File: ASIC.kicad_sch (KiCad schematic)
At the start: 66 parts, among them U10 BM1370_mode1, U11 MCP1824T-1202E/OT, U12 MCP1824T-0802E, U7 SN74AVC4T774, U8 25MHz, U9 BM1370_mode1

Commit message: More BOM cleanup
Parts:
- C38, C54, C55, C56, C57, C58, C59, C60, C61, C62: DK 490-5523-1-ND -> 490-18214-1-ND
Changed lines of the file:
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@@
 			)
 		)
-		(property "DK" "490-5523-1-ND"
+		(property "DK" "490-18214-1-ND"
 			(at 231.14 72.39 0)
 			(effects
@@
 			)
 		)
-		(property "DK" "490-5523-1-ND"
+		(property "DK" "490-18214-1-ND"
 			(at 222.25 72.39 0)
 			(effects
@@
 			)
 		)
-		(property "DK" "490-5523-1-ND"
+		(property "DK" "490-18214-1-ND"
 			(at 240.03 72.39 0)
 			(effects
@@
 			)
 		)
-		(property "DK" "490-5523-1-ND"
+		(property "DK" "490-18214-1-ND"
 			(at 118.11 72.39 0)
 			(effects
@@
 			)
 		)
-		(property "DK" "490-5523-1-ND"
+		(property "DK" "490-18214-1-ND"
 			(at 142.24 72.39 0)
 			(effects
@@
 			)
 		)
-		(property "DK" "490-5523-1-ND"
+		(property "DK" "490-18214-1-ND"
 			(at 109.22 72.39 0)
 			(effects
@@
 			)
 		)
-		(property "DK" "490-5523-1-ND"
+		(property "DK" "490-18214-1-ND"
 			(at 213.36 72.39 0)
 			(effects
@@
 			)
 		)
-		(property "DK" "490-5523-1-ND"
+		(property "DK" "490-18214-1-ND"
 			(at 246.38 72.39 0)
 			(effects
@@
 			)
 		)
-		(property "DK" "490-5523-1-ND"
+		(property "DK" "490-18214-1-ND"
 			(at 127 72.39 0)
 			(effects
@@
 			)
 		)
-		(property "DK" "490-5523-1-ND"
+		(property "DK" "490-18214-1-ND"
 			(at 135.89 72.39 0)
 			(effects

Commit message: change config resistors for TPS546 regulator
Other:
- title: (none) -> Bitaxe Gamma Turbo
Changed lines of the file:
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@@
 	(generator "eeschema")
 	(generator_version "8.0")
-	(paper "A4")
+	(paper "A3")
+	(title_block
+		(title "Bitaxe Gamma Turbo")
+		(rev "800")
+	)
 	(junction
 		(at 127 68.58)

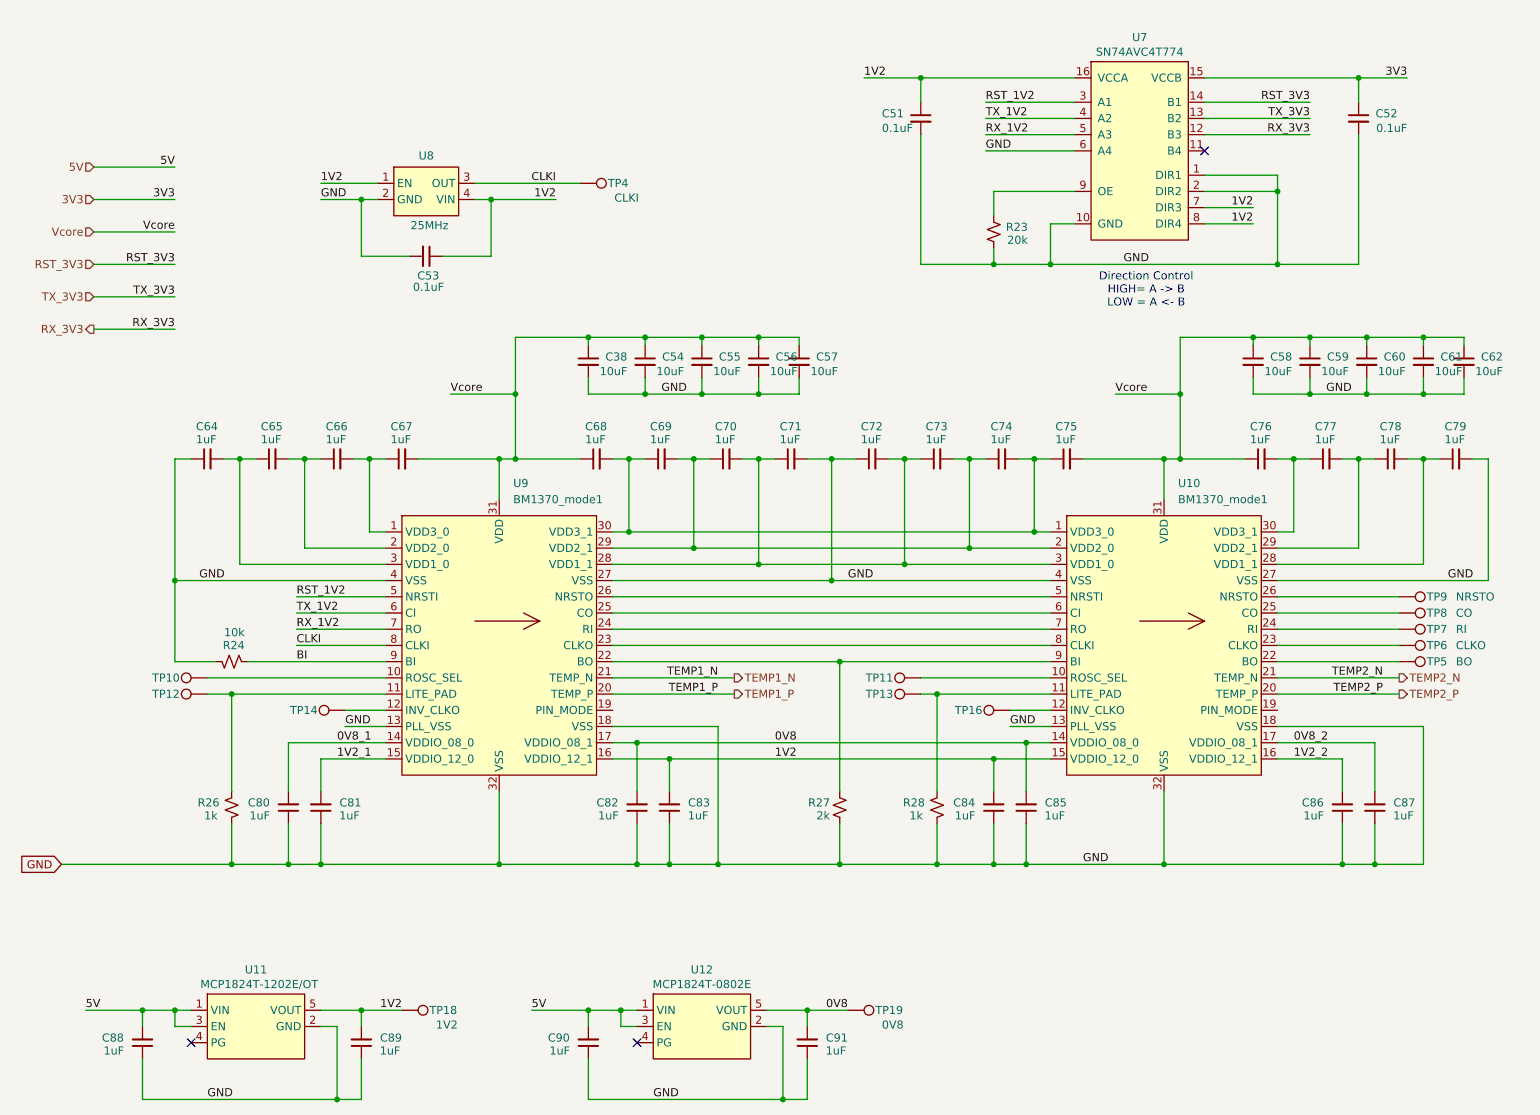
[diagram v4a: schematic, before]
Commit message: cleaned up worksheets
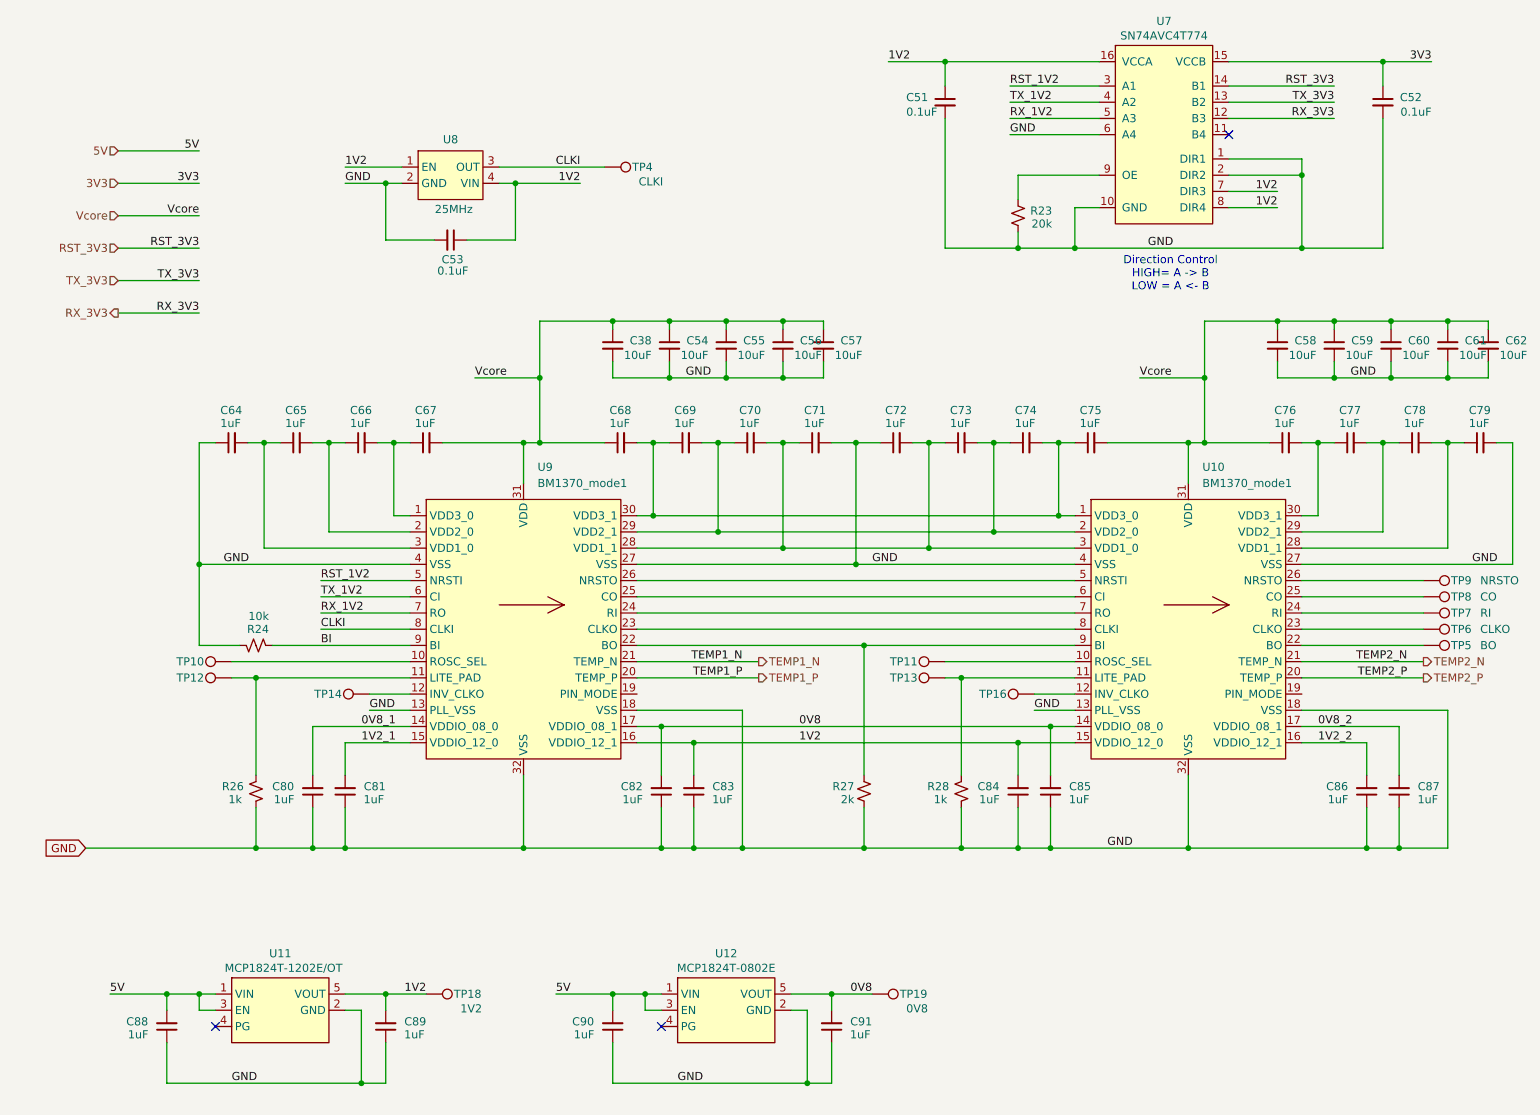
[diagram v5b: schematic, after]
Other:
- moved on the sheet: C38, C51, C52, C53, C54, C55, C56, C57, C58, C59, C60, C61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

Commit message: schematic and track cleanup
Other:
- title: Bitaxe Gamma Turbo -> bitaxeGamma Turbo
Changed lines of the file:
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@@
 	(paper "A4")
 	(title_block
-		(title "Bitaxe Gamma Turbo")
+		(title "bitaxeGamma Turbo")
 		(date "2025-02-28")
 		(rev "800xx")
